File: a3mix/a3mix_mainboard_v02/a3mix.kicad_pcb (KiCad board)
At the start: 4 copper layers, 184.2 x 270.5 mm, 185 parts, among them U5 Teensy4.1

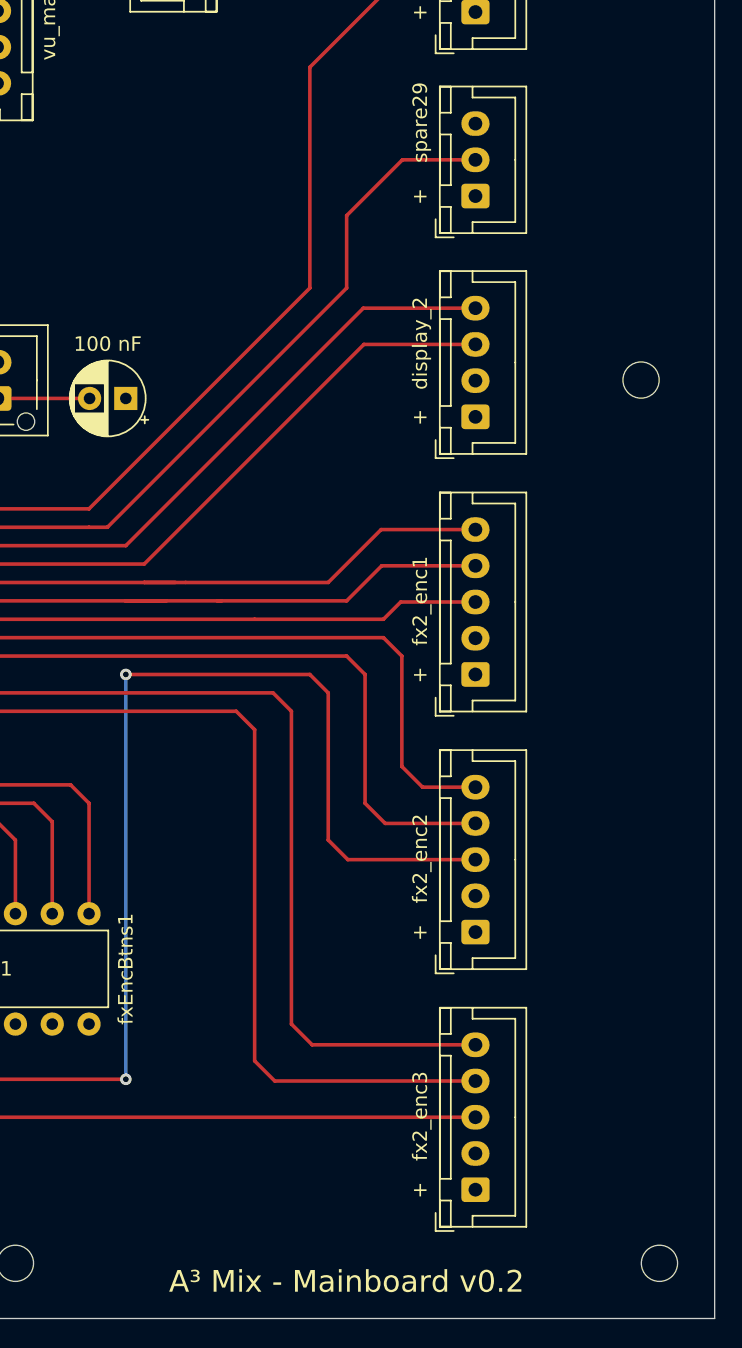
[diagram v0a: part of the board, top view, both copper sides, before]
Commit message: A³ Mix draft license ohl-s
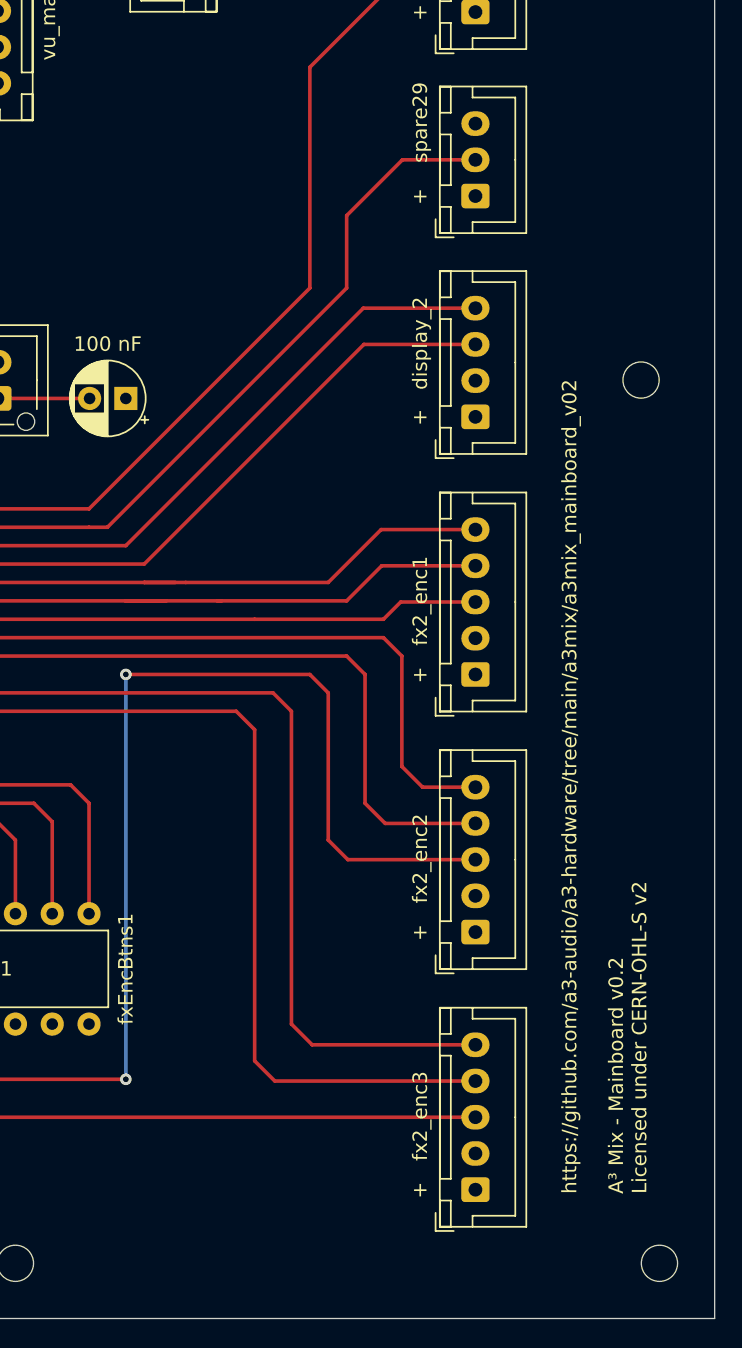
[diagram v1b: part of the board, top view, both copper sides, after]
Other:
- board text added: "https://github.com/a3-audio/a3-hardware/tree/main/a3mix/a3mix_mainboard_v02 A³ Mix - Mainboard v0.2 Licensed under CERN-OHL-S v2"
- board text removed: "A³ Mix - Mainboard v0.2"
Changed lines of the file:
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@@
     (rev "v0.2")
     (company "A3 Audio UG (haftungsbeschränkt)")
+    (comment 3 "https://github.com/a3-audio/a3-hardware")
+    (comment 4 "Licensed under CERN-OHL-S v2")
   )
   (layers
@@
     (effects (font (size 1 1) (thickness 0.15)))
   )
-  (gr_text "A³ Mix - Mainboard v0.2" (at 171.45 280.67) (layer "F.SilkS")
-    (effects (font (size 1.5 1.5) (thickness 0.3)))
+  (gr_text "https://github.com/a3-audio/a3-hardware/tree/main/a3mix/a3mix_mainboard_v02\n\nA³ Mix - Mainboard v0.2\nLicensed under CERN-OHL-S v2\n" (at 189.251893 274.609318 90) (layer "F.SilkS")
+    (effects (font (size 1 1) (thickness 0.1)) (justify left))
   )
   (gr_text "+" (at 39.37 137.16) (layer "F.SilkS")
